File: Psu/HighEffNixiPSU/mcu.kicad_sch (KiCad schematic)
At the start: 26 parts, among them J2 USB_C_Receptacle_USB2.0, SW1 EN, SW2 EN, U3 ESP32-S3-MINI-1U, U4 TPS562202

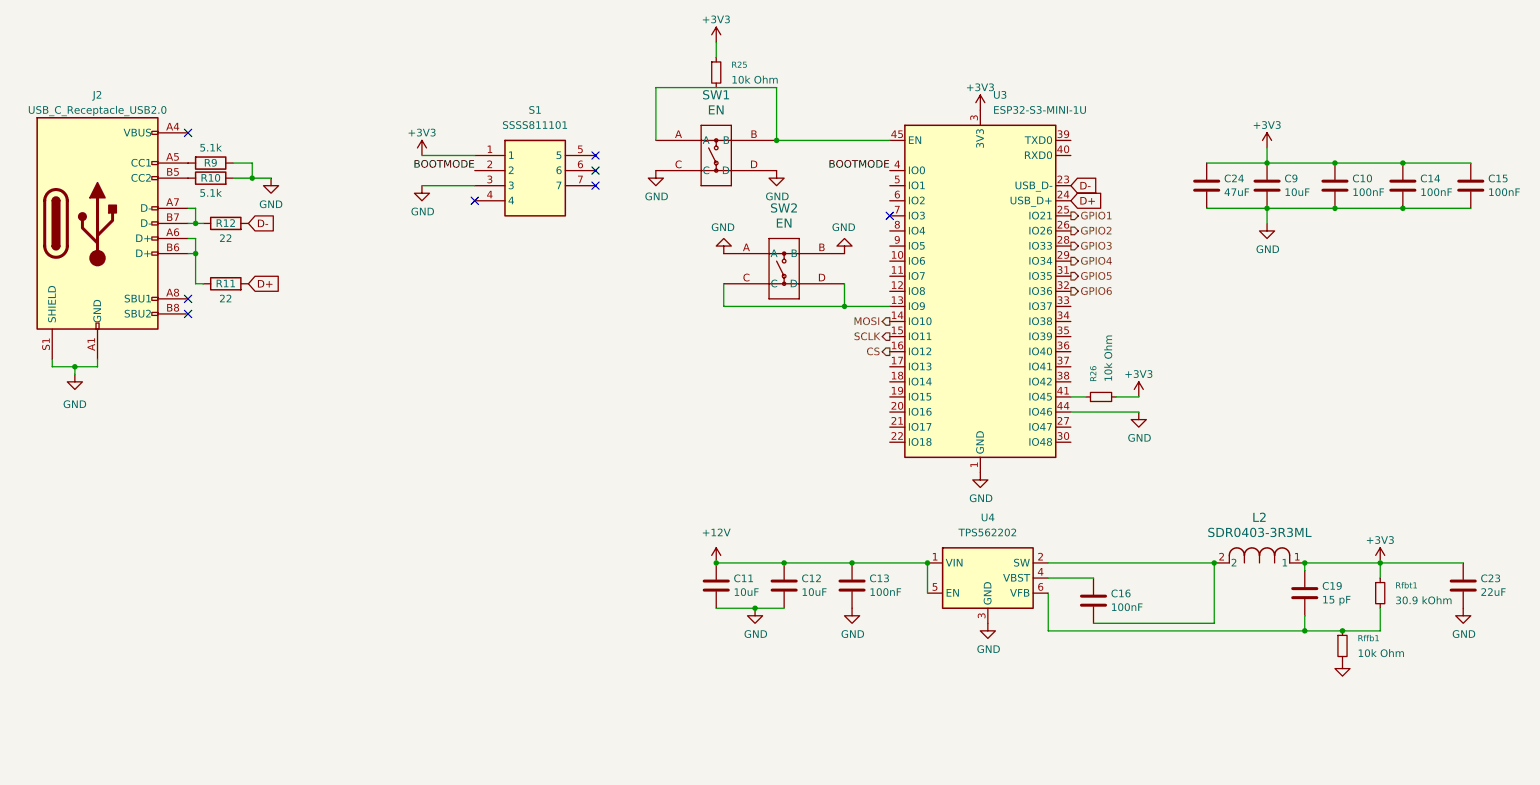
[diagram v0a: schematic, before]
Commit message: FPGA time
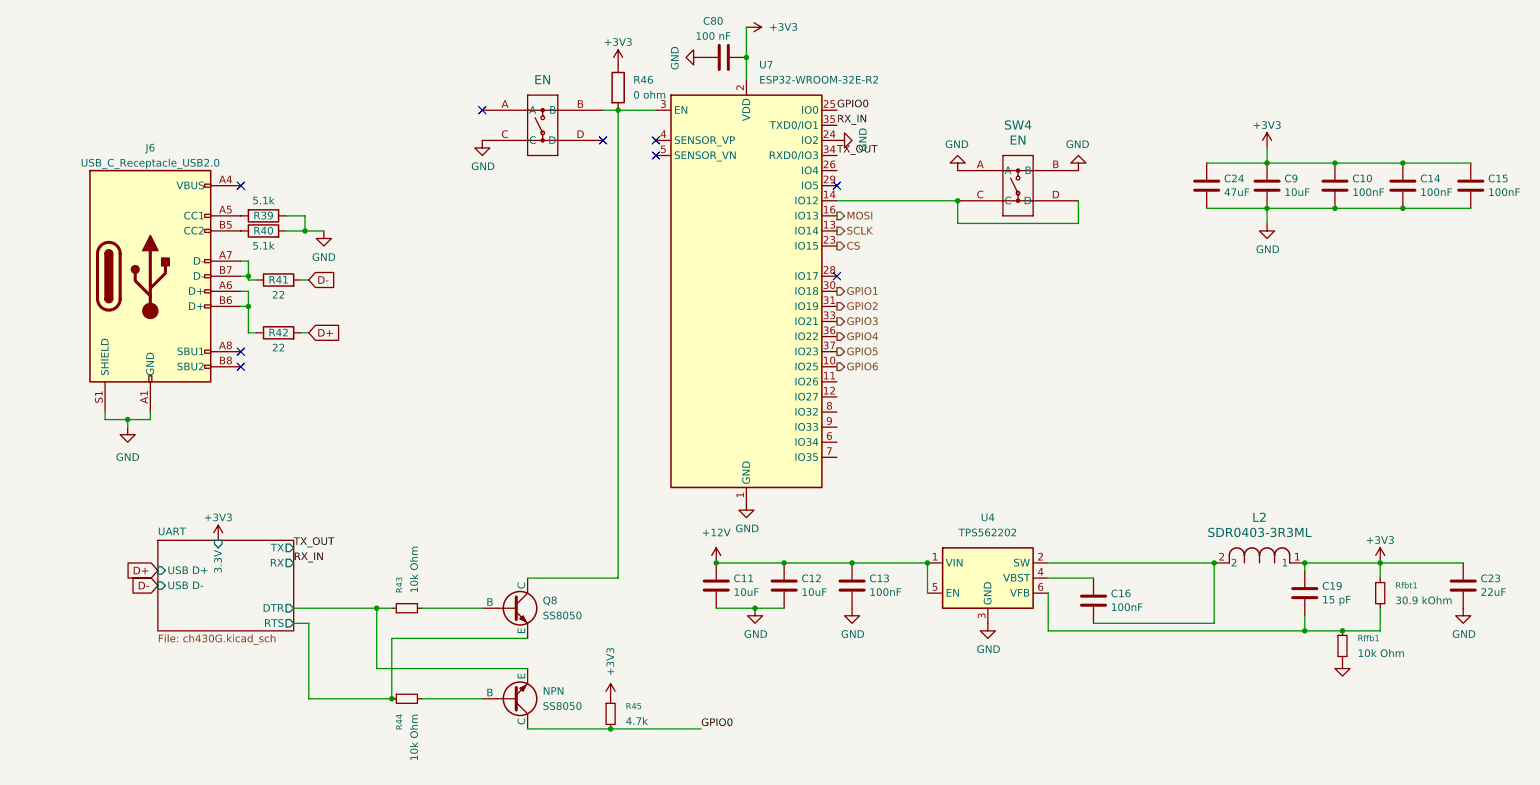
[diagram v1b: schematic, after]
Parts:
- removed J2: USB_C_Receptacle_USB2.0, Connector_USB:USB_C_Receptacle_HRO_TYPE-C-31-M-12, symbol Connector:USB_C_Receptacle_USB2.0
- removed R10, R9: 5.1k, Resistor_SMD:R_0603_1608Metric, symbol Device:R
- removed R11, R12: 22, Resistor_SMD:R_0603_1608Metric, symbol Device:R
- removed R25, R26: 10k Ohm, Resistor_SMD:R_0603_1608Metric, symbol Device:R_Small
- removed S1: SSSS811101, footprints:SSSS811101, symbol Personal:SSSS811101
- removed SW1, SW2: EN, footprints:KH-6X6X5H-STM_SKE, symbol 2026-02-17_13-05-37:KH-6X6X5H-STM
- removed U3: ESP32-S3-MINI-1U, RF_Module:ESP32-S2-MINI-1U, symbol RF_Module:ESP32-S3-MINI-1U
- added C80: 100 nF, Capacitor_SMD:C_0805_2012Metric, symbol Device:C
- added J6: USB_C_Receptacle_USB2.0, Connector_USB:USB_C_Receptacle_HRO_TYPE-C-31-M-12, symbol Connector:USB_C_Receptacle_USB2.0
- added Q8: SS8050, Package_TO_SOT_SMD:SOT-23, symbol Simulation_SPICE:NPN
- added R39, R40: 5.1k, Resistor_SMD:R_0805_2012Metric, symbol Device:R
- added R41, R42: 22, Resistor_SMD:R_0805_2012Metric, symbol Device:R
- added R43, R44: 10k Ohm, Resistor_SMD:R_0805_2012Metric, symbol Device:R_Small
- added R45: 4.7k, Resistor_SMD:R_0603_1608Metric, symbol Device:R_Small
- added R46: 0 ohm, Resistor_SMD:R_0805_2012Metric, symbol Device:R
- added SS8050: NPN, Package_TO_SOT_SMD:SOT-23, symbol Simulation_SPICE:NPN
- added SW3, SW4: EN, footprints:KH-6X6X5H-STM_SKE, symbol 2026-02-17_13-05-37:KH-6X6X5H-STM
- added U7: ESP32-WROOM-32E-R2, RF_Module:ESP32-WROOM-32D, symbol RF_Module:ESP32-WROOM-32E-R2
- C11, C12: LCSC C1691 -> C92487
- C19: LCSC C1804 -> C107110
- C23: LCSC C441864 -> C45783
- Rffb1: LCSC Part # C2930027 -> C25804
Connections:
- net +3V3: now also C80.1, R45.1, R46.1, U7.2 (VDD)
- net CS: now also U7.23 (IO15)
- net D+: now also R42.2
- net D-: now also R41.2
- net GND: now also C80.2, J6.A1 (GND), J6.A12 (GND), J6.B1 (GND), J6.B12 (GND), J6.S1 (SHIELD), R39.1, R40.2, SW3.C, SW4.A, SW4.B, U7.1 (GND), U7.15 (GND), U7.24 (IO2), U7.38 (GND), U7.39 (GND)
- net GPIO1: now also U7.30 (IO18)
- net GPIO2: now also U7.31 (IO19)
- net GPIO3: now also U7.33 (IO21)
- net GPIO4: now also U7.36 (IO22)
- net GPIO5: now also U7.37 (IO23)
- net GPIO6: now also U7.10 (IO25)
- net MOSI: now also U7.16 (IO13)
- net SCLK: now also U7.13 (IO14)
- new net: SW4.C, SW4.D, U7.14 (IO12)
- new net: Q8.1 (C), R46.2, SW3.B, U7.3 (EN)
- new net: J6.B5 (CC2), R40.1
- new net: J6.A4 (VBUS), J6.A9 (VBUS), J6.B4 (VBUS), J6.B9 (VBUS)
- new net: J6.A5 (CC1), R39.2
- new net: J6.A6 (D+), J6.B6 (D+), R42.1
- new net: J6.A7 (D-), J6.B7 (D-), R41.1
- new net: Q8.2 (B), R43.2
- new net: R44.2, SS8050.2 (B)
- new net GPIO0: R45.2, SS8050.1 (C), U7.25 (IO0)
- new net RX_IN: U7.35 (TXD0/IO1)
- new net TX_OUT: U7.34 (RXD0/IO3)
- new net UART/DTR: R43.1, SS8050.3 (E)
- new net UART/RTS: Q8.3 (E), R44.1
- no-connect marks 8 -> 9
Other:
- added sheet UART (ch430G.kicad_sch)
